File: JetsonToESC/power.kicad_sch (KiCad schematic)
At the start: 10 parts, among them U3 LMR51420XDDCR

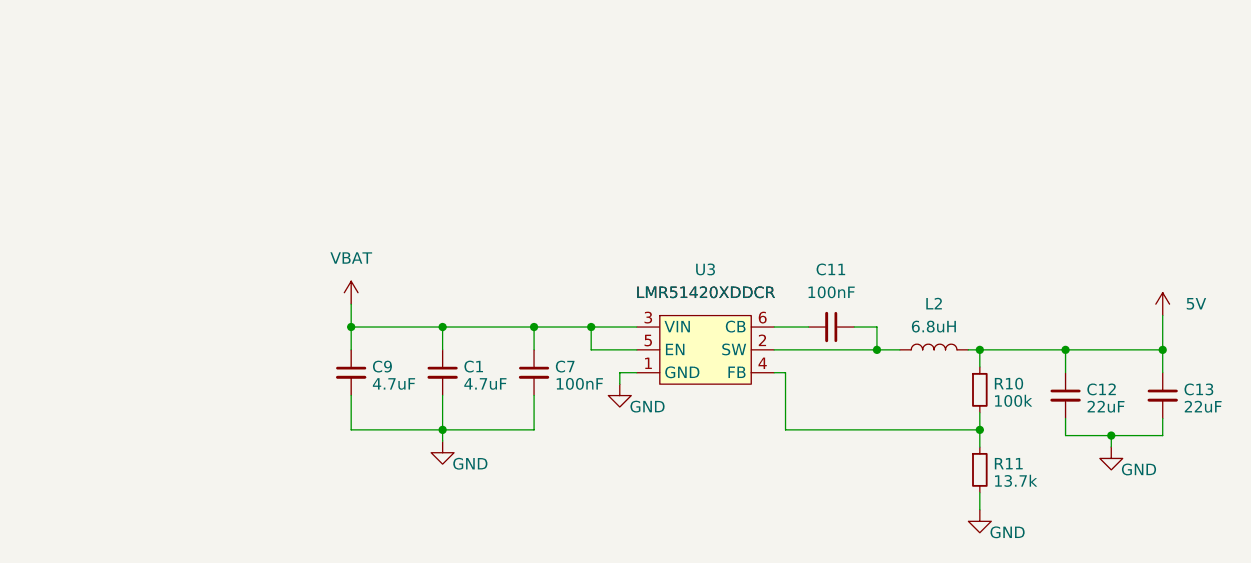
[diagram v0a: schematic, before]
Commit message: Start On this Branch
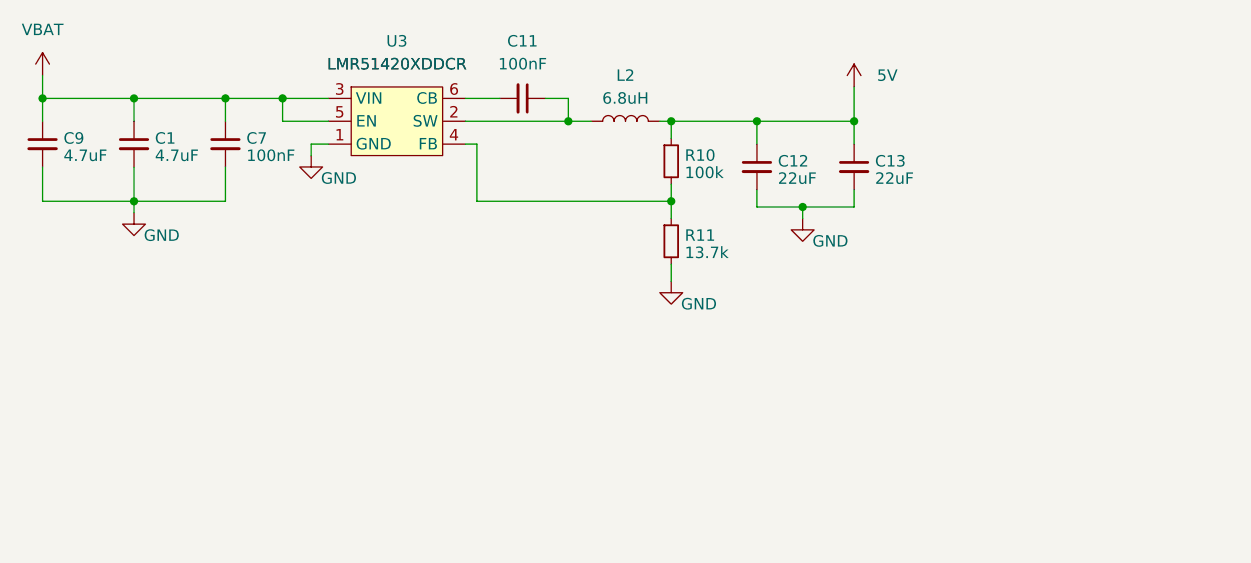
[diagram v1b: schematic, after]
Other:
- moved on the sheet: C1, C11, C12, C13, C7, C9, L2, R10, R11, U3

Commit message: Work on current sense and io expansion branch
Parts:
- C11, C7: footprint Capacitor_SMD:C_0805_2012Metric_Pad1.18x1.45mm_HandSolder -> Capacitor_SMD:C_0603_1608Metric
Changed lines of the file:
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@@
 			)
 		)
-		(property "Footprint" "Capacitor_SMD:C_0805_2012Metric_Pad1.18x1.45mm_HandSolder"
+		(property "Footprint" "Capacitor_SMD:C_0603_1608Metric"
 			(at 110.49 63.5 0)
 			(effects
@@
 			)
 		)
-		(property "Footprint" "Capacitor_SMD:C_0805_2012Metric_Pad1.18x1.45mm_HandSolder"
+		(property "Footprint" "Capacitor_SMD:C_0603_1608Metric"
 			(at 77.47 68.58 0)
 			(effects
